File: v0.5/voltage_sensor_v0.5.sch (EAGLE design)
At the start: 64 parts, among them IC1 AP2112K-3.3TRG1, J1 1017505, J2 20020316-H021B01LF, J9 RJ11-6, M1 MOV-14D431KTR, M2 MOV-14D431KTR, M3 MOV-14D431KTR, T1 ZMPT101B, T2 ZMPT101B, T3 ZMPT101B

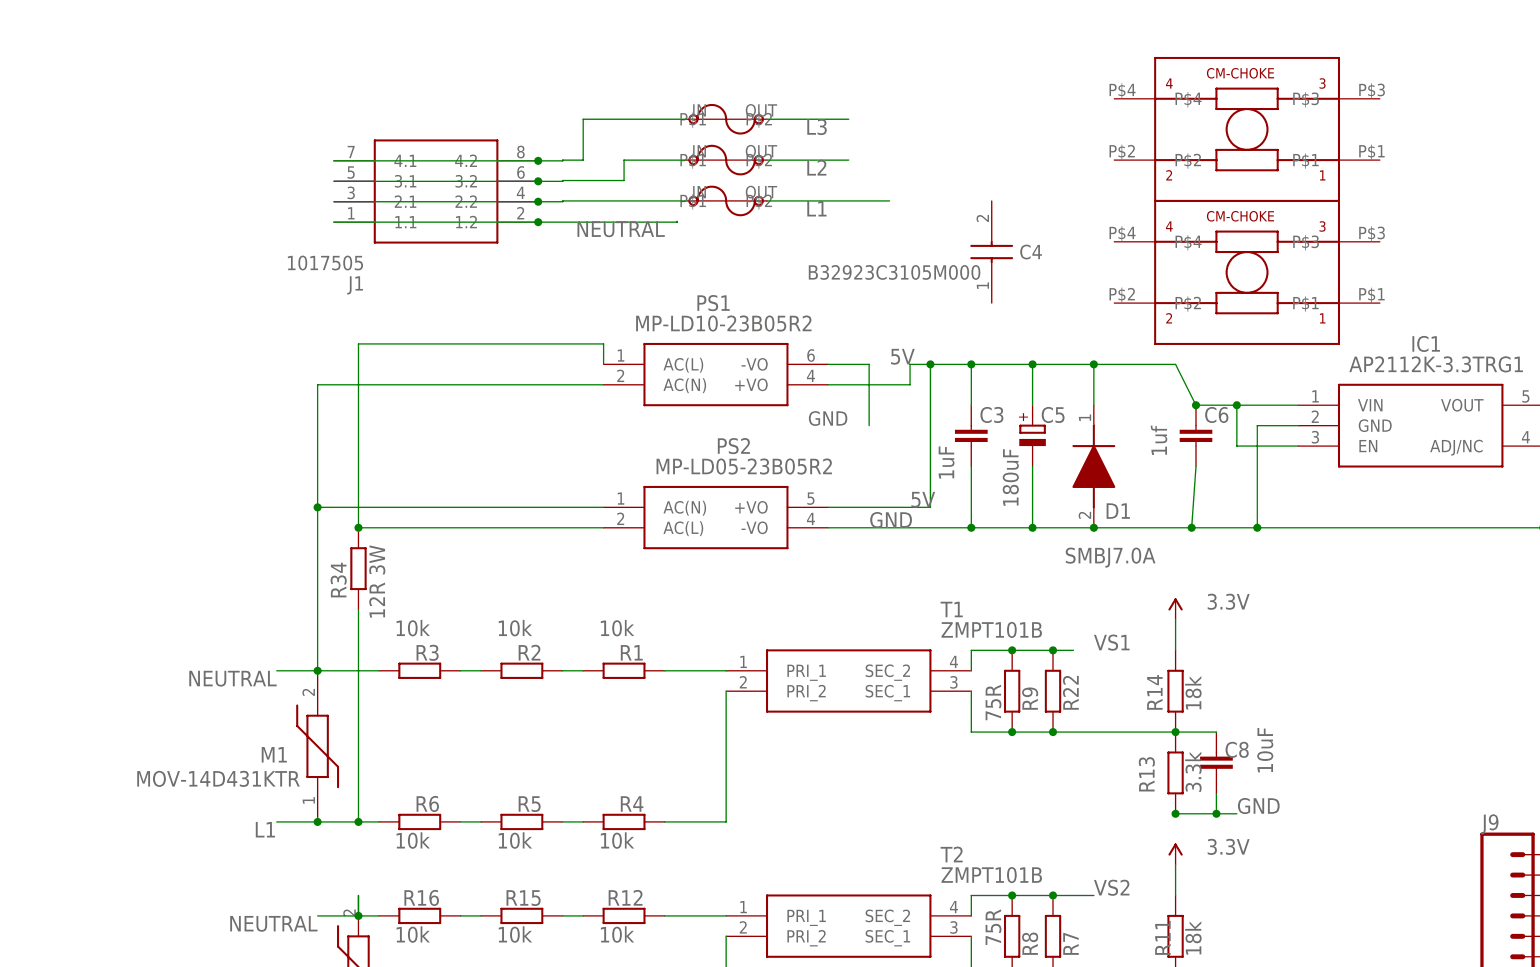
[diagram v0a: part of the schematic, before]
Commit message: new design
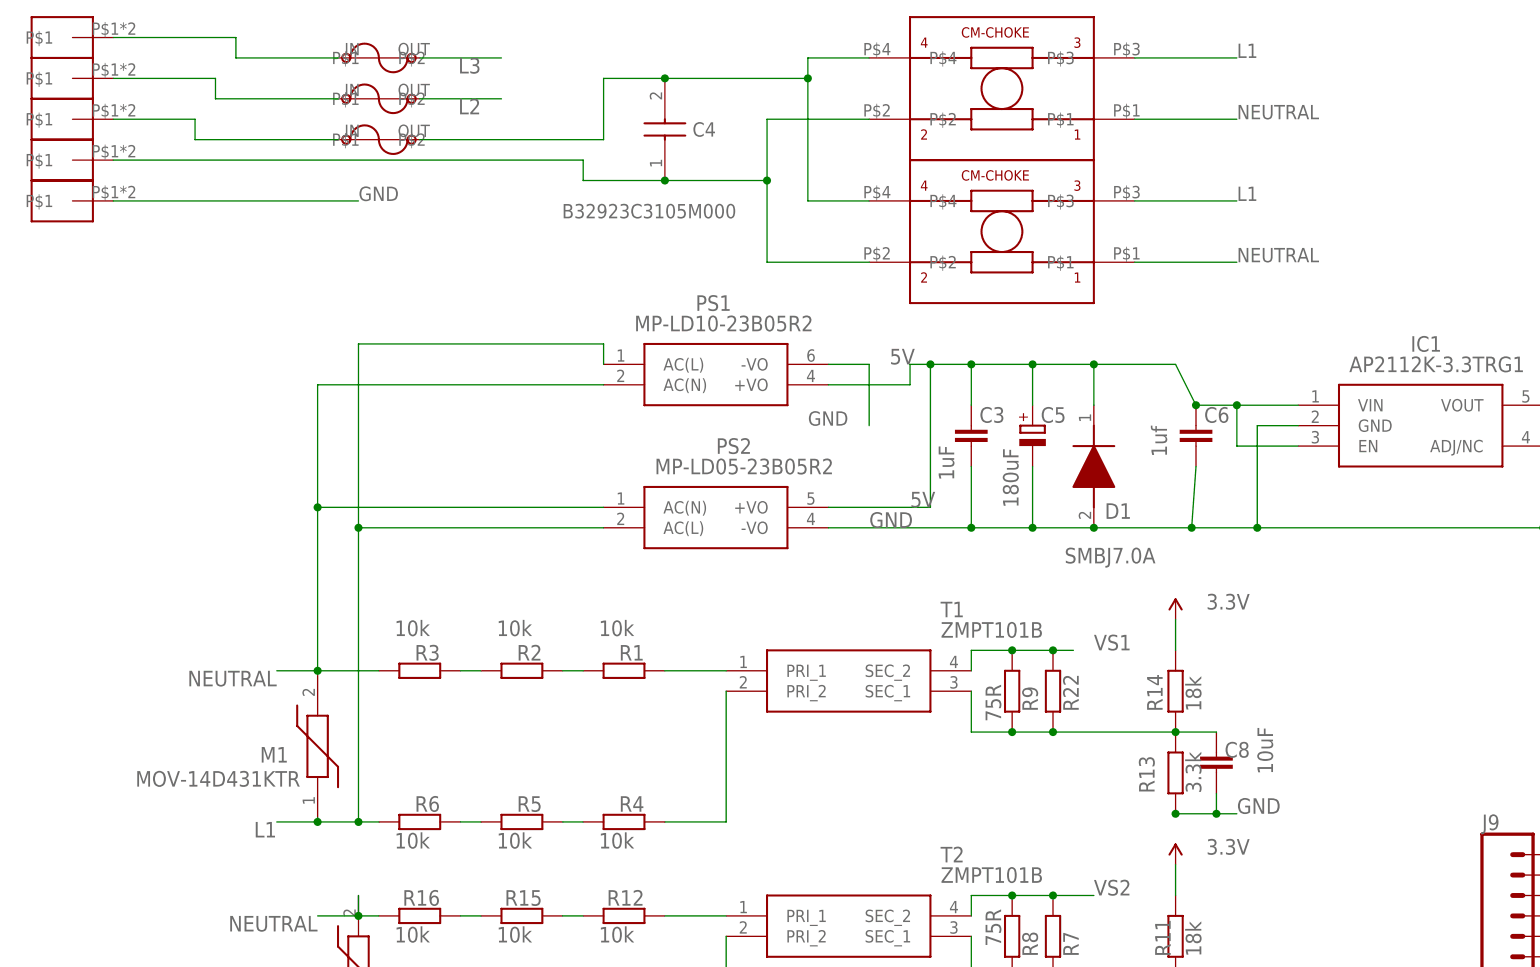
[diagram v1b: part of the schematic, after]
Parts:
- removed J1: 1017505, 1017505:1017505
- removed R34: 12R 3W, rcl:R-EU_R2512
- added U$3, U$5, U$6, U$7, U$8: 1905010, Phoenix-Contact-1905010:1905010
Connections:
- net GND: now also U$7.P$1
- net L1: now also PS1.AC(L), PS2.AC(L), U$1.P$3, U$2.P$3; no longer F1.P$1, R34.1
- net N$16: now also U$8.P$1; no longer J1.4.1, J1.4.2
- net N$17: now also C4.2, F1.P$1, U$1.P$4, U$2.P$4; no longer PS1.AC(L), PS2.AC(L), R34.2
- net N$7: now also U$5.P$1; no longer J1.2.1, J1.2.2
- net N$8: now also U$3.P$1; no longer J1.3.1, J1.3.2
- net NEUTRAL: now also C4.1, U$1.P$1, U$1.P$2, U$2.P$1, U$2.P$2, U$6.P$1; no longer J1.1.1, J1.1.2
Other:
- moved on the sheet: C4

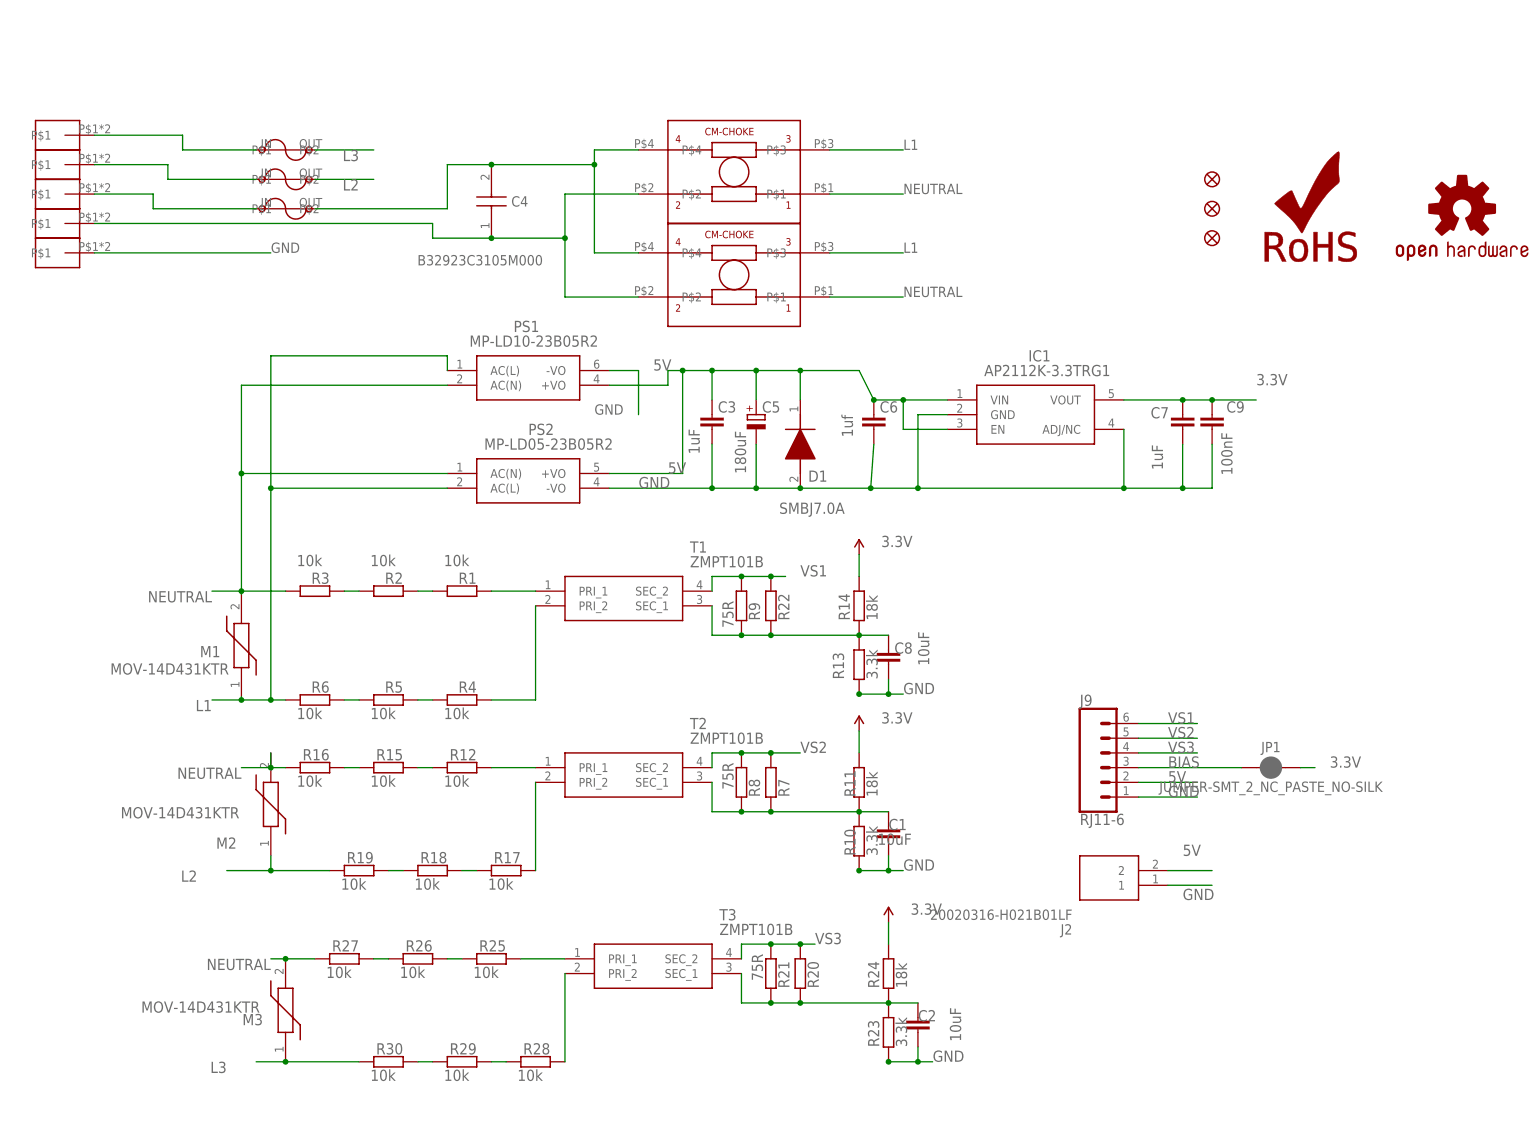
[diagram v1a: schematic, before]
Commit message: finish layout
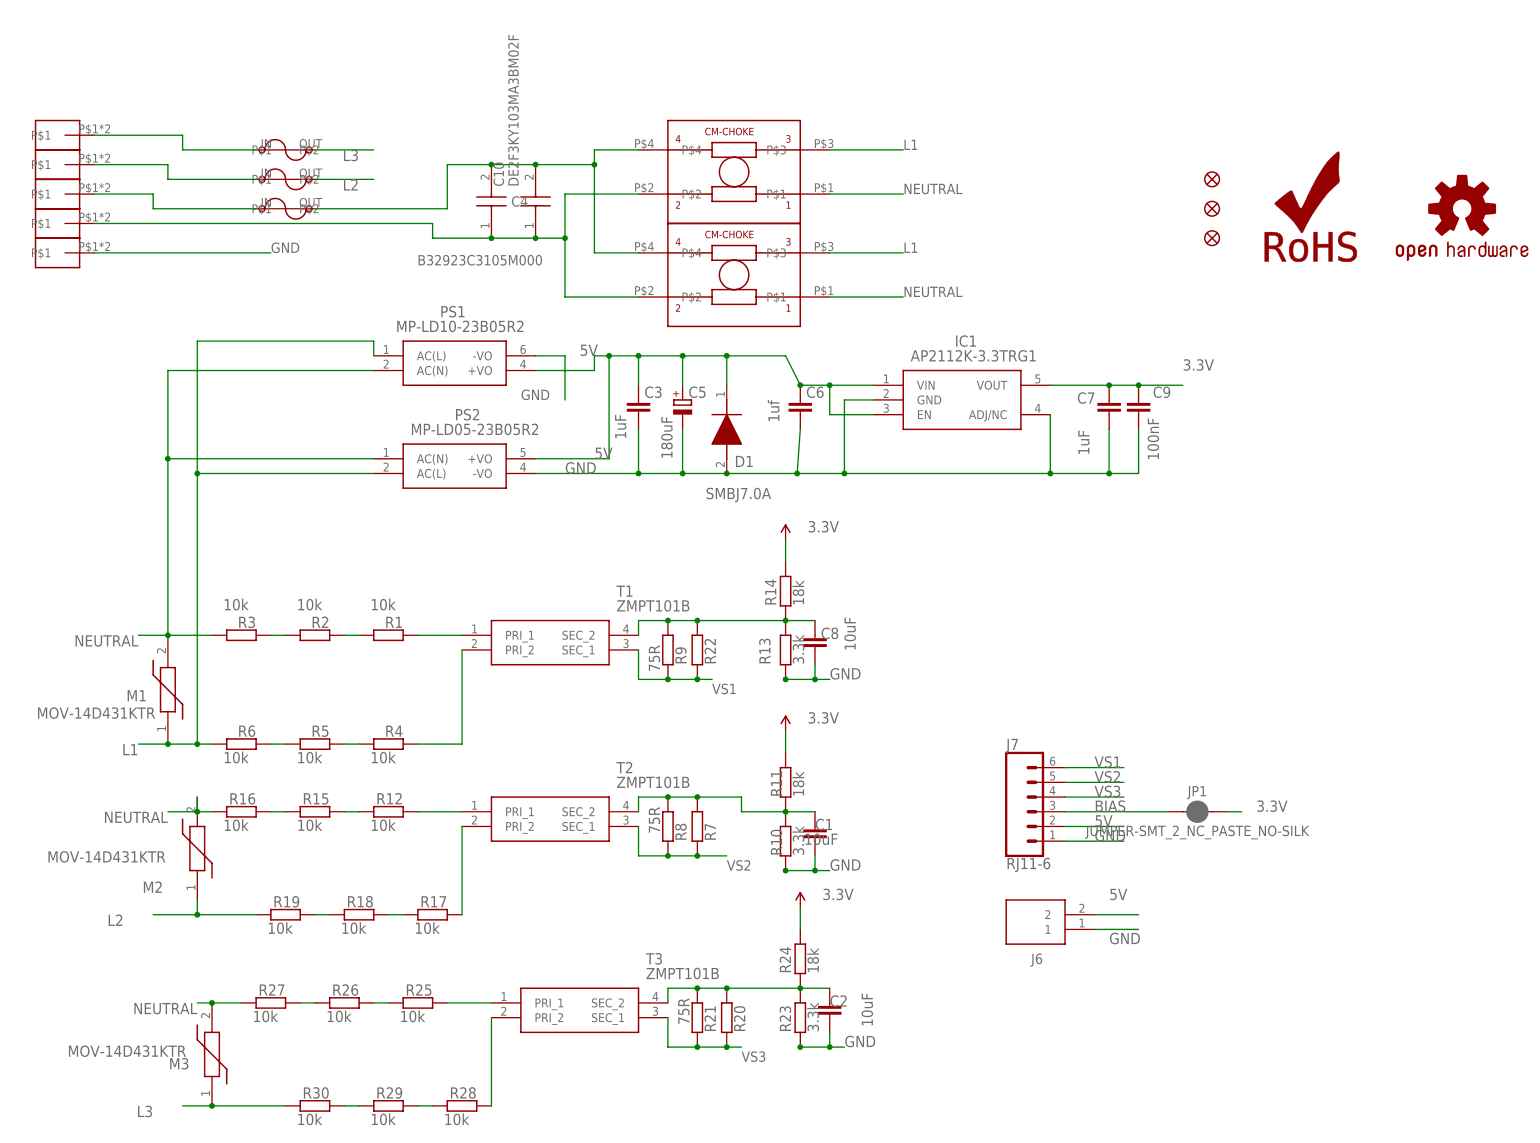
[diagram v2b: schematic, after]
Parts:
- removed J2: 20020316-H021B01LF, 20020316-H021B01LF:20020316-H021B01LF
- removed J9: RJ11-6, SparkFun-Connectors:RJ11-6
- added C10: DE2F3KY103MA3BM02F, DE2F3KY103MA3BM02F:DE2F3KY103MA3BM02F
- added J6: 20020316-H021B01LF, 20020316-H021B01LF:20020316-H021B01LF
- added J7: RJ11-6, SparkFun-Connectors:RJ11-6
- renumbered U$3 to J4, U$5 to J3, U$7 to J1, U$8 to J5
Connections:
- removed net N$18: C2.1, R20.1, R21.1, R23.1, R24.1, T3.SEC_1
- new net N$26: C8.1, R13.1, R14.1, R22.2, R9.2, T1.SEC_2
- net 5V: now also J6.2, J7.2; no longer J2.2, J9.2
- net BIAS: now also J7.3; no longer J9.3
- net GND: now also J6.1, J7.1; no longer J2.1, J9.1
- net N$17: now also C10.2
- net N$25: now also C2.1, R20.2, R21.2, R23.1, R24.1, T3.SEC_2; no longer C8.1, R13.1, R14.1, R22.1, R9.1, T1.SEC_1
- net N$9: now also R7.2, R8.2, T2.SEC_2; no longer R7.1, R8.1, T2.SEC_1
- net NEUTRAL: now also C10.1
- net VS1: now also J7.6, R22.1, R9.1, T1.SEC_1; no longer J9.6, R22.2, R9.2, T1.SEC_2
- net VS2: now also J7.5, R7.1, R8.1, T2.SEC_1; no longer J9.5, R7.2, R8.2, T2.SEC_2
- net VS3: now also J7.4, R20.1, R21.1, T3.SEC_1; no longer J9.4, R20.2, R21.2, T3.SEC_2
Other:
- moved on the sheet: C1, C2, C3, C5, C6, C7, C8, C9, D1, IC1, JP1, M1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
